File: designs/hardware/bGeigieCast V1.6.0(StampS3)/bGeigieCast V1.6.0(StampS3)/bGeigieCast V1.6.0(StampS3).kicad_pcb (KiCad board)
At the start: 2 copper layers, 24.8 x 27.4 mm, 3 parts, among them J1 Left, J2 Right, U2 XBEE-socket

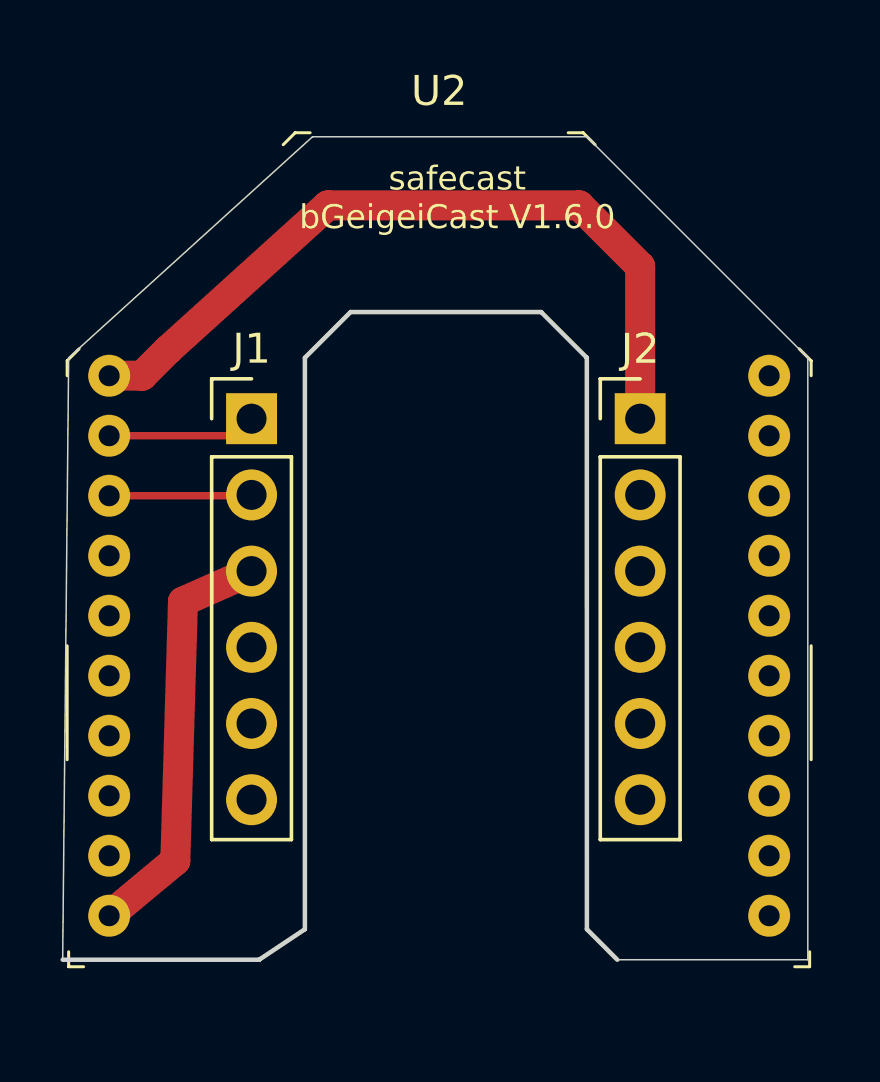
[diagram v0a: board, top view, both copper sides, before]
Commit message: Added V1.6.2 Gerbers and many boards updates.
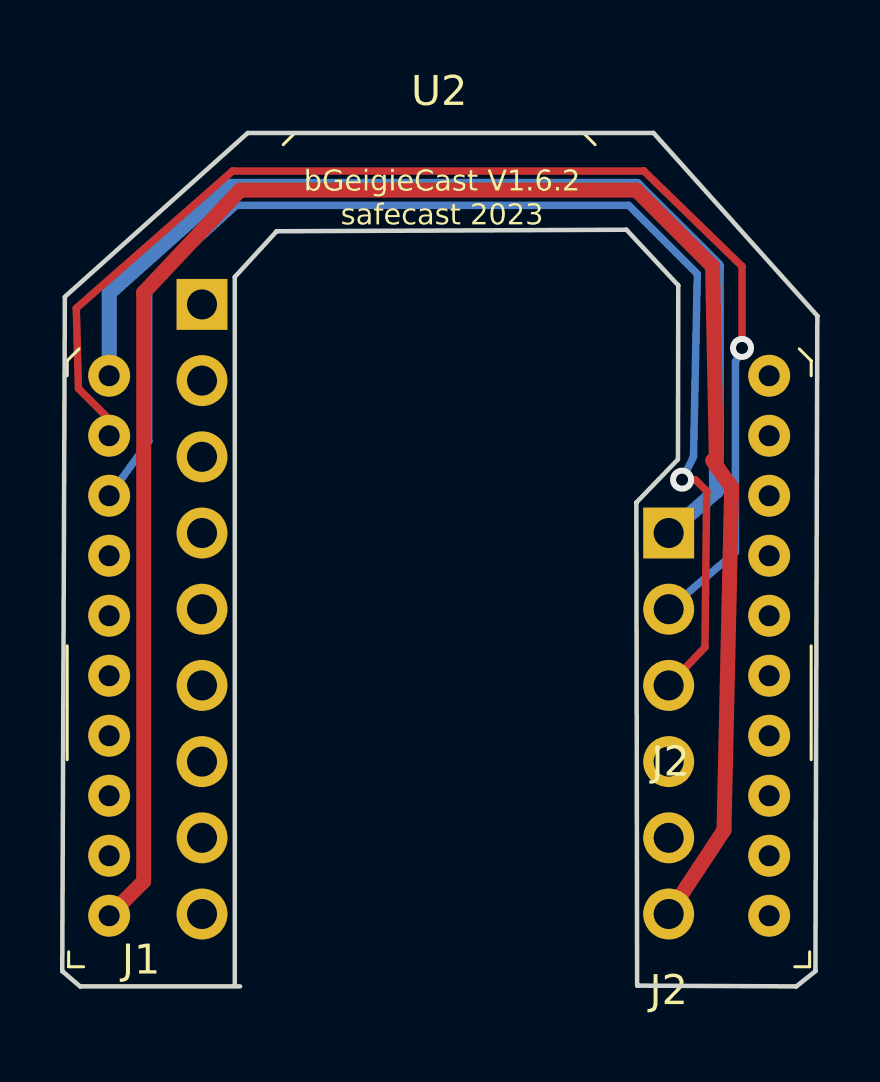
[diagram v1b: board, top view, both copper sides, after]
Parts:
- J1: footprint Connector_PinHeader_2.54mm:PinHeader_1x06_P2.54mm_Vertical -> Connector_PinHeader_2.54mm:PinHeader_1x09_P2.54mm_Vertical
- moved J1 4.15 mm to (140.5, 97.0)
- moved J2 3.93 mm to (156.1, 104.6)
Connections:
- net Net-(J2-Pin_7) renamed +3.3V
- J1 pad 1: Net-(J1-Pin_6) -> unconnected-(J1-Pin_6-Pad1)
- J1 pad 2: Net-(J1-Pin_5) -> unconnected-(J1-Pin_5-Pad2)
- J1 pad 3: Net-(J1-Pin_4) -> unconnected-(J1-Pin_4-Pad3)
- J2 pad 12: unconnected-(J2-Pin_12-Pad12) -> GND
- J2 pad 8: unconnected-(J2-Pin_8-Pad8) -> Net-(J2-Pin_8)
- J2 pad 9: unconnected-(J2-Pin_9-Pad9) -> Net-(J2-Pin_9)
- U2 pad 10: Net-(J1-Pin_4) -> GND
- U2 pad 2: Net-(J1-Pin_6) -> Net-(J2-Pin_8)
- U2 pad 3: Net-(J1-Pin_5) -> Net-(J2-Pin_9)
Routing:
- net GND: track 0.00 -> 65.3 mm
- net Net-(J2-Pin_8): track 0.00 -> 43.2 mm, vias 0 -> 1
- net Net-(J2-Pin_9): track 0.00 -> 42.6 mm, vias 0 -> 1
- net Net-(J1-Pin_4): track 14.0 -> 0.00 mm
- net +3.3V: track 25.8 -> 35.1 mm
- net Net-(J1-Pin_6): track 4.98 -> 0.00 mm
- net Net-(J1-Pin_5): track 4.80 -> 0.00 mm
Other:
- board size 24.8 x 27.4 mm -> 25.2 x 28.4 mm
- board text added: "bGeigieCast V1.6.2 safecast 2023"
- board text removed: "safecast bGeigeiCast V1.6.0"
